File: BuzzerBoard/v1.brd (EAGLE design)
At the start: 100 x 80 mm, 9 parts, among them J1 p0, U1 LM386MX-1/NOPB

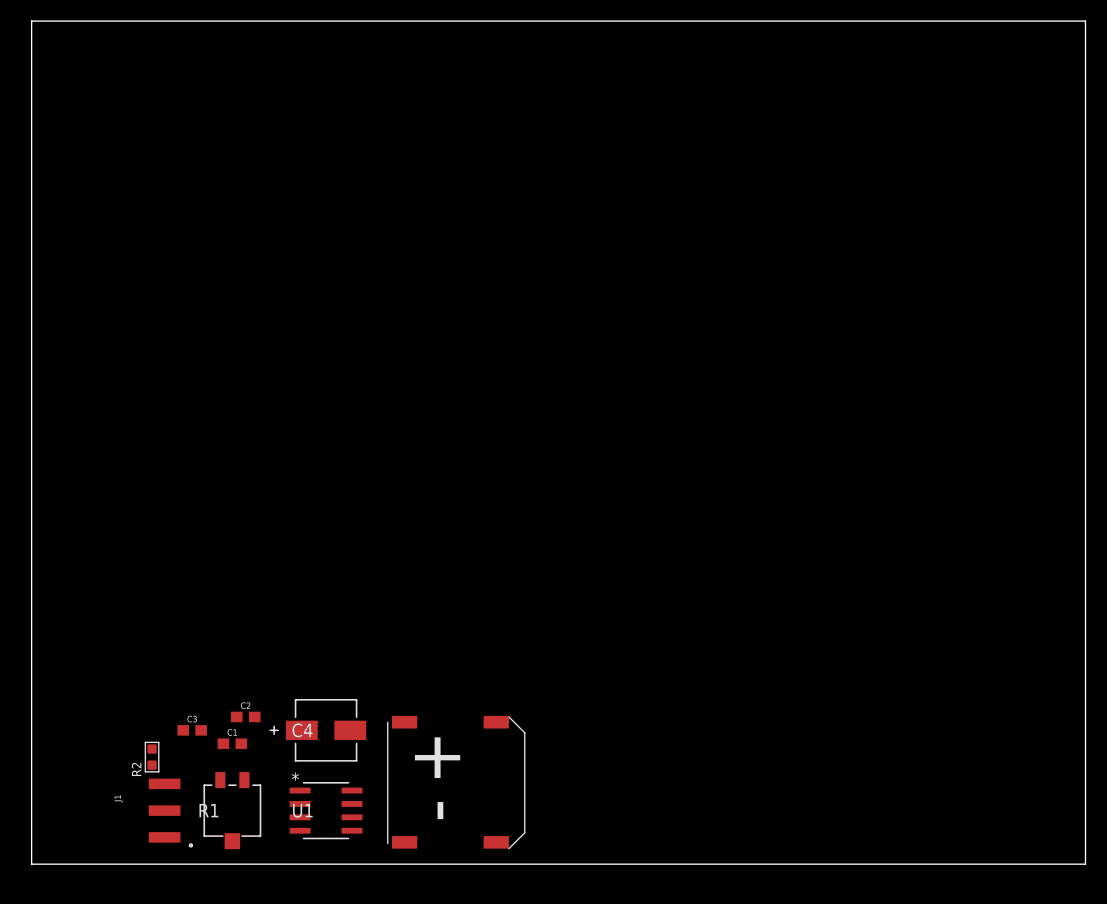
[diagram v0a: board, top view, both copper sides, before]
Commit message: V1 to OSH park.
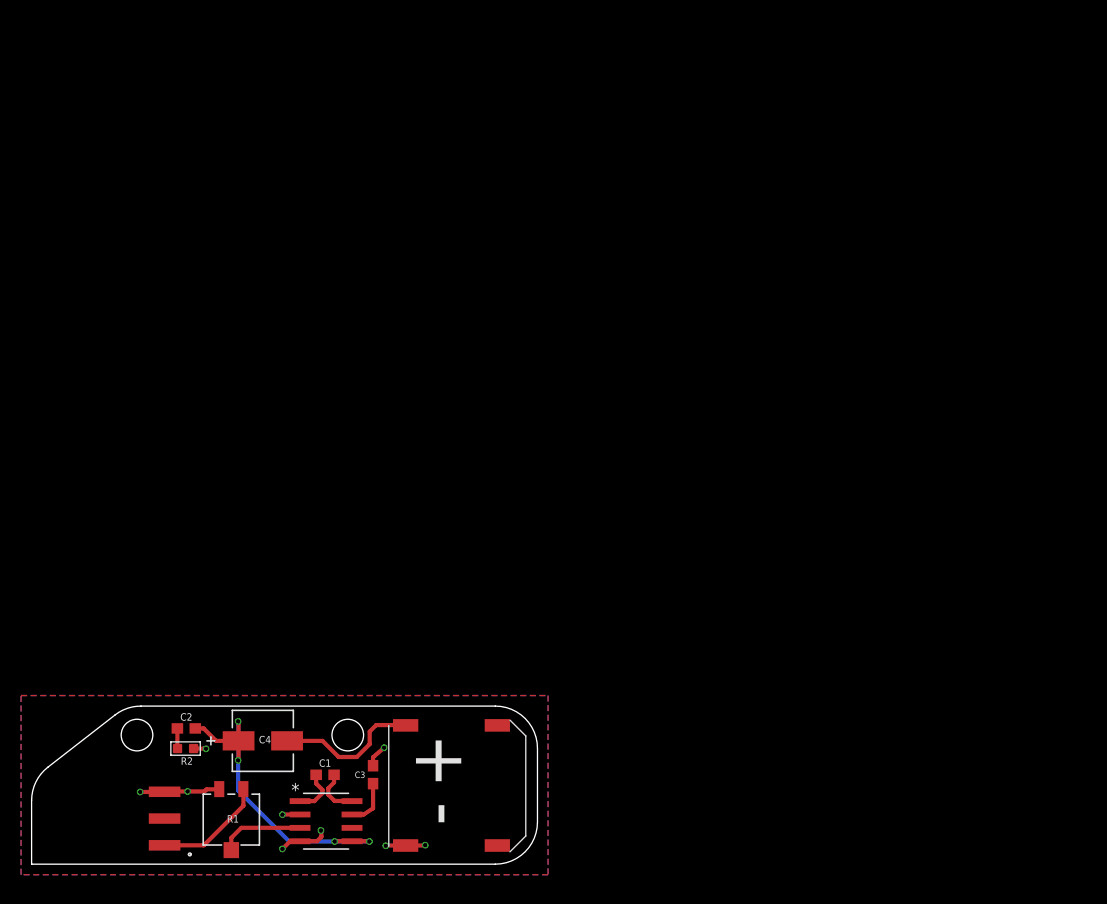
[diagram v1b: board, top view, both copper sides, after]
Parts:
- added U$2: (no value), boneyard:32BITS_LOGO
- moved C3 17.7 mm to (32.4, 8.49), turned to 90 degrees
- moved C1 9.28 mm to (27.9, 8.48)
- moved C4 6.08 mm to (21.9, 11.7)
- moved C2 5.74 mm to (14.7, 12.9), turned to 180 degrees
- moved R2 3.28 mm to (14.6, 11.0), turned to 270 degrees
- moved U1 1.00 mm to (27.9, 4.08)
- moved R1 0.86 mm to (18.9, 4.23)
- moved J1 0.75 mm to (7.62, 4.33)
- moved U$1 0.32 mm to (34.4, 13.7)
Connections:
- net N$3 renamed VOUT
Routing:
- net VOUT: track 0.00 -> 32.7 mm, vias 0 -> 4
- net GND: track 0.00 -> 21.3 mm, vias 0 -> 9
- net +: track 0.00 -> 13.9 mm
- net P0: track 0.00 -> 10.6 mm
- net IN+: track 0.00 -> 8.09 mm
- net GAIN: track 0.00 -> 4.61 mm
- net BYPASS: track 0.00 -> 4.51 mm
- net N$2: track 0.00 -> 4.42 mm
- net N$1: track 0.00 -> 1.92 mm
- added copper zone on layer 1, net 3.3V
- added copper zone on layer 16, net GND
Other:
- board size 100 x 80 mm -> 48 x 15 mm
- board text added: "Moto:Bit Speaker v1.0 | 32bits.io"
